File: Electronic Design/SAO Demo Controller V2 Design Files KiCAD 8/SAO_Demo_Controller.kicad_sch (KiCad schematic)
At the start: 10 parts, among them U1 RP2040-Zero, X1 SAO_conn, X2 SAO_conn, X5 QWIIC, X6 QWIIC

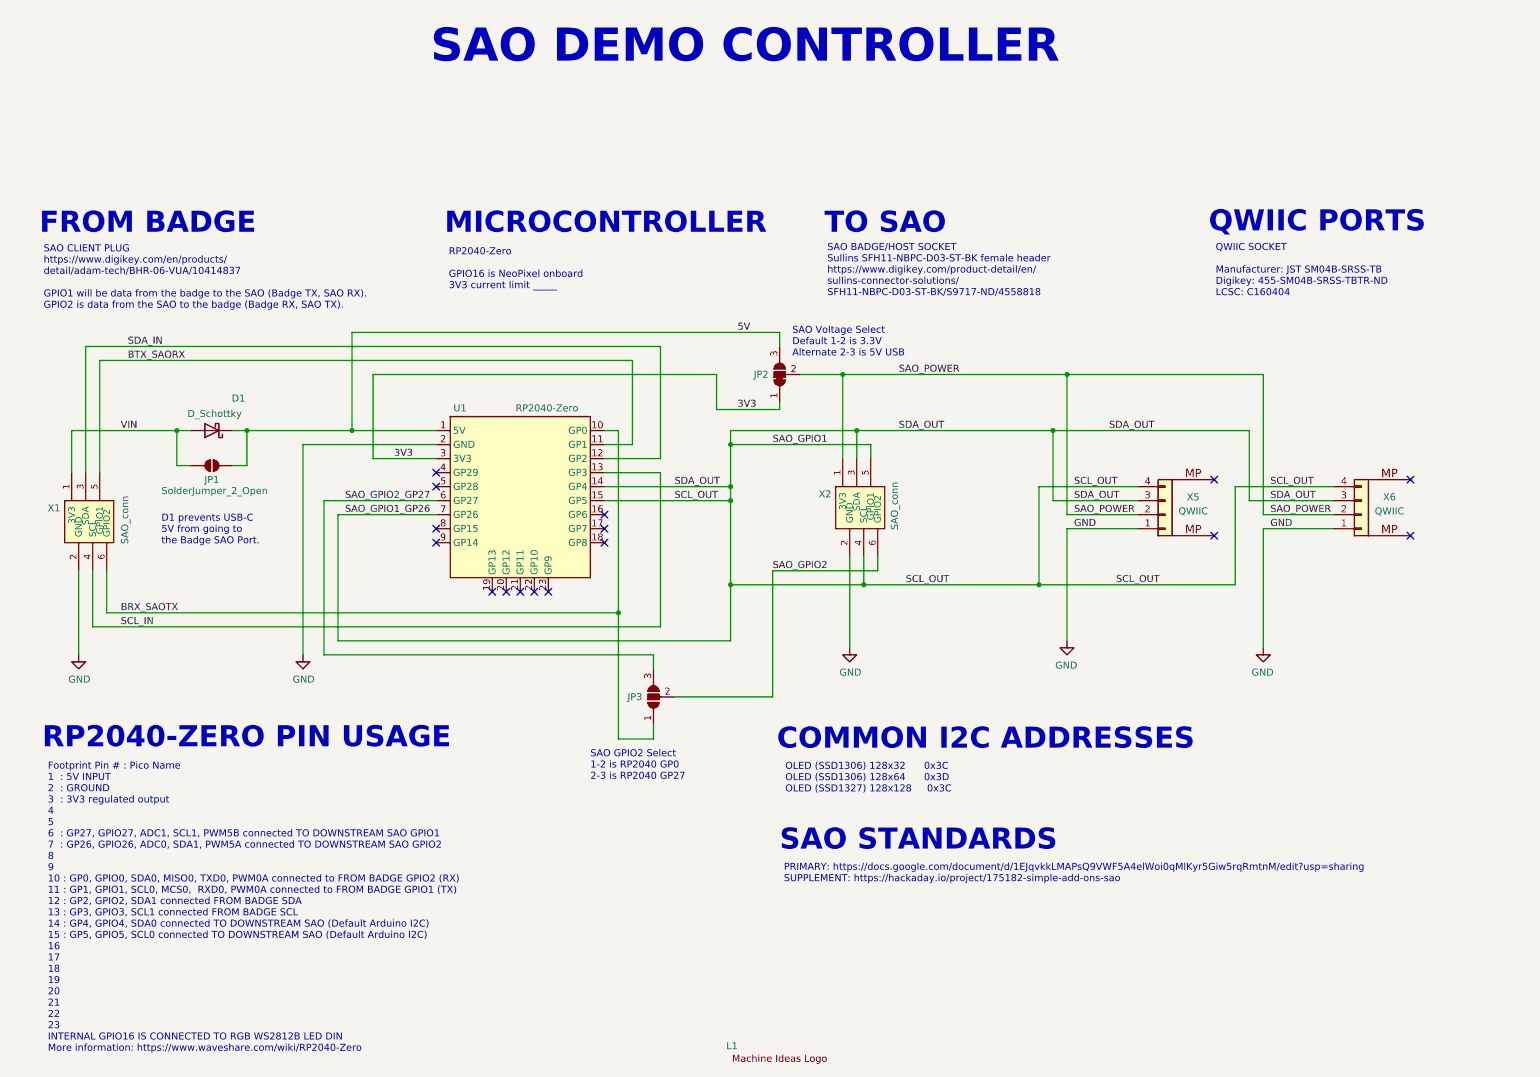
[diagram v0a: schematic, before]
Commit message: Update V2 schematics, docs, renders
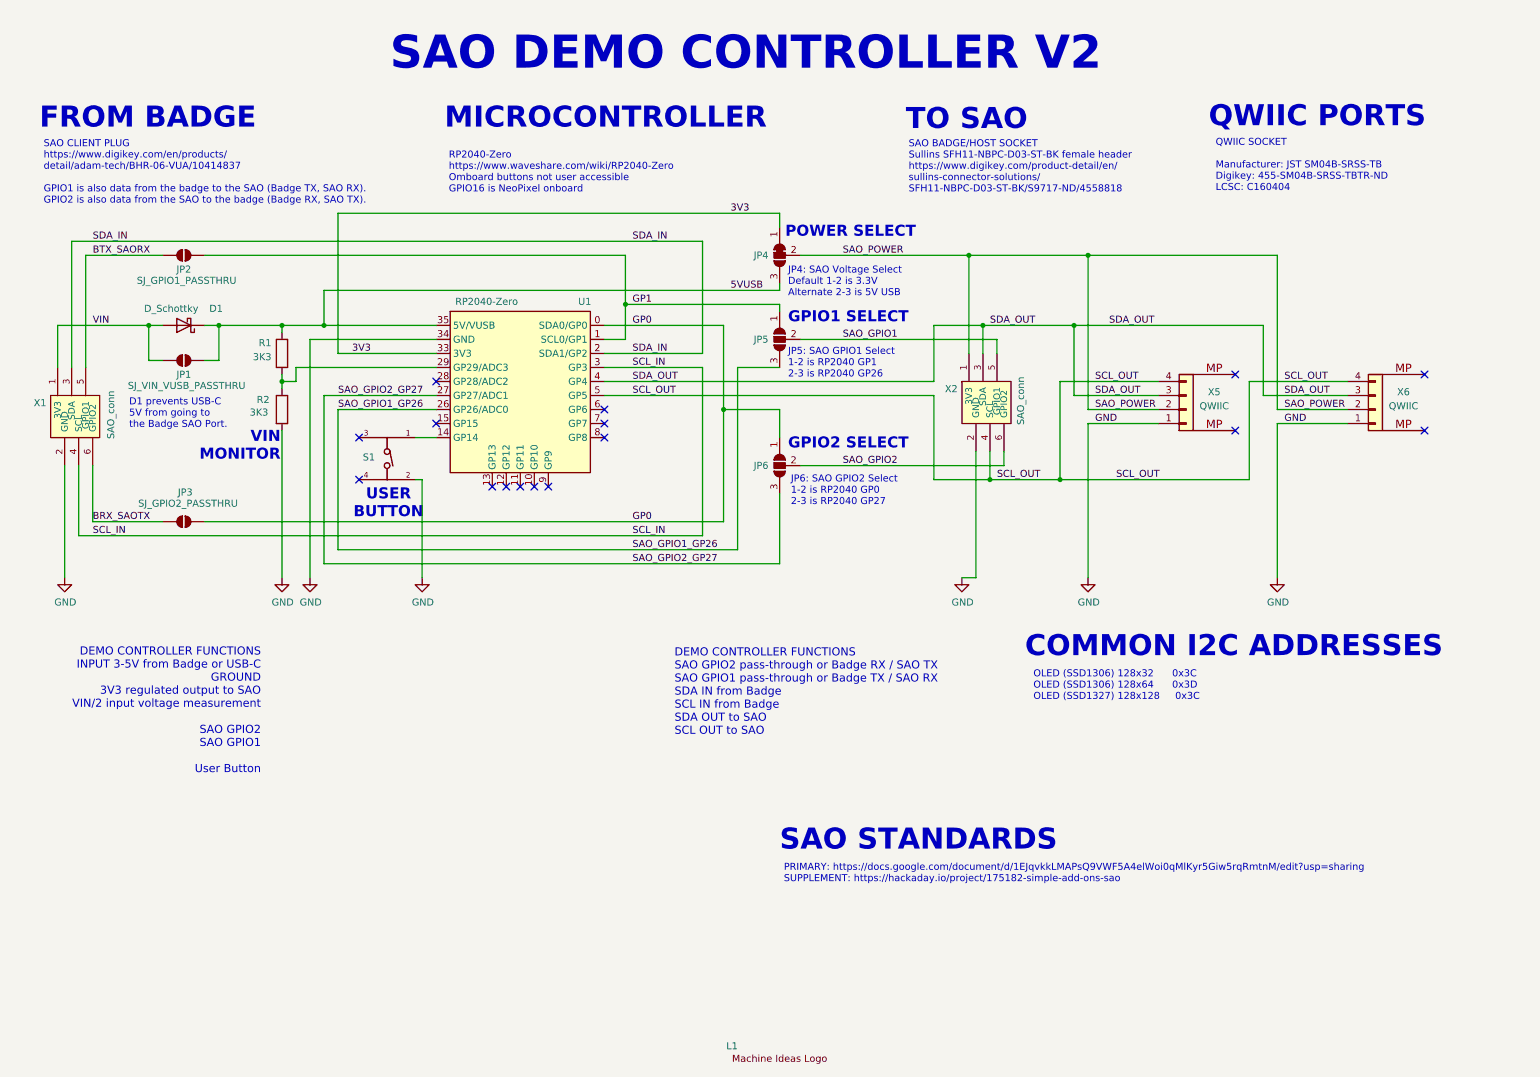
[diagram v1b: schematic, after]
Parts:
- added JP2: SJ_GPIO1_PASSTHRU, Jumper:SolderJumper-2_P1.3mm_Open_RoundedPad1.0x1.5mm, symbol Jumper:SolderJumper_2_Open
- added JP3: SJ_GPIO2_PASSTHRU, Jumper:SolderJumper-2_P1.3mm_Open_RoundedPad1.0x1.5mm, symbol Jumper:SolderJumper_2_Open
- added JP5: SolderJumper_3_Open, Jumper:SolderJumper-3_P1.3mm_Open_RoundedPad1.0x1.5mm_NumberLabels, symbol Jumper:SolderJumper_3_Open
- added R1, R2: 3K3, Resistor_SMD:R_0805_2012Metric, symbol Device:R
- added S1: 434331045822, Andy_Footprint_Library:Button_Wurth_4343X10458XX, symbol ANDY_SYMBOL_LIBRARY:Button_Wurth_434331045822
- JP1: value SolderJumper_2_Open -> SJ_VIN_VUSB_PASSTHRU
- U1: symbol ANDY_SYMBOL_LIBRARY:RP2040-Zero -> ANDY_SYMBOL_LIBRARY:RP2040-Zero-Andy
- renumbered JP2 to JP4, JP3 to JP6
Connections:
- net 3V3: now also U1.33 (3V3); no longer U1.3 (3V3)
- net BRX_SAOTX: now also JP3.1 (A); no longer JP6.1 (A), U1.10 (GP0)
- net BTX_SAORX: now also JP2.1 (A); no longer U1.11 (GP1)
- net GND: now also U1.34 (GND), R2.2, S1.2; no longer U1.2 (GND)
- net SAO_GPIO1: now also JP5.2 (C); no longer U1.14 (GP4), U1.15 (GP5), U1.7 (GP26), X2.3 (SDA), X2.4 (SCL), X5.3 (Pin_3), X5.4 (Pin_4), X6.3 (Pin_3), X6.4 (Pin_4)
- net SAO_GPIO2_GP27: now also U1.27 (GP27/ADC1); no longer U1.6 (GP27)
- net SCL_IN: now also U1.3 (GP3); no longer U1.13 (GP3)
- net SDA_IN: now also U1.2 (SDA1/GP2); no longer U1.12 (GP2)
- net SDA_OUT: now reaches U1.4 (GP4)
- net SDA_OUT: now also X2.3 (SDA), X5.3 (Pin_3), X6.3 (Pin_3)
- net SCL_OUT: now reaches U1.5 (GP5)
- net SCL_OUT: now also X2.4 (SCL), X5.4 (Pin_4), X6.4 (Pin_4)
- net 5V renamed 5VUSB
- net 5VUSB: now also U1.35 (5V/VUSB), R1.2; no longer U1.1 (5V)
- new net: S1.1, U1.14 (GP14)
- new net: R1.1, R2.1, U1.29 (GP29/ADC3)
- new net GP0: JP3.2 (B), JP6.1 (A), U1.0 (SDA0/GP0)
- new net GP1: JP2.2 (B), JP5.1 (A), U1.1 (SCL0/GP1)
- new net SAO_GPIO1_GP26: JP5.3 (B), U1.26 (GP26/ADC0)
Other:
- note added: "DEMO CONTROLLER FUNCTIONS INPUT 3-5V from Badge or USB-C GROUND 3V3 regulated output to SAO VIN/2 input voltage measurement SAO GPIO2 SAO GPIO1 User Button"
- note added: "DEMO CONTROLLER FUNCTIONS SAO GPIO2 pass-through or Badge RX / SAO TX SAO GPIO1 pass-through or Badge TX / SAO RX SDA IN from Badge SCL IN from Badge SDA OUT to SAO SCL OUT to SAO"
- note added: "GPIO1 SELECT"
- note added: "GPIO2 SELECT"
- note added: "JP4: SAO Voltage Select Default 1-2 is 3.3V Alternate 2-3 is 5V USB"
- note added: "JP5: SAO GPIO1 Select 1-2 is RP2040 GP1 2-3 is RP2040 GP26"
- note added: "JP6: SAO GPIO2 Select 1-2 is RP2040 GP0 2-3 is RP2040 GP27"
- note added: "POWER SELECT"
- note added: "RP2040-Zero https://www.waveshare.com/wiki/RP2040-Zero Omboard buttons not user accessible GPIO16 is NeoPixel onboard"
- note added: "SAO CLIENT PLUG https://www.digikey.com/en/products/ detail/adam-tech/BHR-06-VUA/10414837 GPIO1 is also data from the badge to the SAO (Badge TX, SAO RX). GPIO2 is also data from the SAO to the badge (Badge RX, SAO TX)."
- note added: "SAO DEMO CONTROLLER V2"
- note added: "USER BUTTON"
- note added: "VIN MONITOR"
- note removed: "Footprint Pin # : Pico Name 1 : 5V INPUT 2 : GROUND 3 : 3V3 regulated output 4 5 6 : GP27, GPIO27, ADC1, SCL1, PWM5B connected TO DOWNSTREAM SAO GPIO1 7 : GP26, GPIO26, ADC0, SDA1, PWM5A connected TO DOWNSTREAM SAO GPIO2 8 9 10 : GP0, GPIO0, SDA0, MISO0, TXD0, PWM0A connected to FROM BADGE GPIO2 (RX) 11 : GP1, GPIO1, SCL0, MCS0, RXD0, PWM0A connected to FROM BADGE GPIO1 (TX) 12 : GP2, GPIO2, SDA1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"
- note removed: "RP2040-ZERO PIN USAGE"
- note removed: "RP2040-Zero GPIO16 is NeoPixel onboard 3V3 current limit _____"
- note removed: "SAO CLIENT PLUG https://www.digikey.com/en/products/ detail/adam-tech/BHR-06-VUA/10414837 GPIO1 will be data from the badge to the SAO (Badge TX, SAO RX). GPIO2 is data from the SAO to the badge (Badge RX, SAO TX)."
- note removed: "SAO DEMO CONTROLLER"
- note removed: "SAO GPIO2 Select 1-2 is RP2040 GP0 2-3 is RP2040 GP27"
- note removed: "SAO Voltage Select Default 1-2 is 3.3V Alternate 2-3 is 5V USB"
- moved on the sheet: D1, JP1, JP4, JP6, U1, X1, X2, X5, X6
